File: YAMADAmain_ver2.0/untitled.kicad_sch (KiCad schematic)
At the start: 18 parts, among them J10 RX==RX, J11 TX==TX, J8 RX==TX, J9 TX==RX, U14 4.7k, U15 SW_DP3T, U16 0.1u, U18 STM32F446RETx-stm32, U19 0.1u, U20 0.1u, U22 0.1u, U23 0.1u, U3 0.1u, U4 D_Schottky, U7 4.7u, U9 ST-LINK

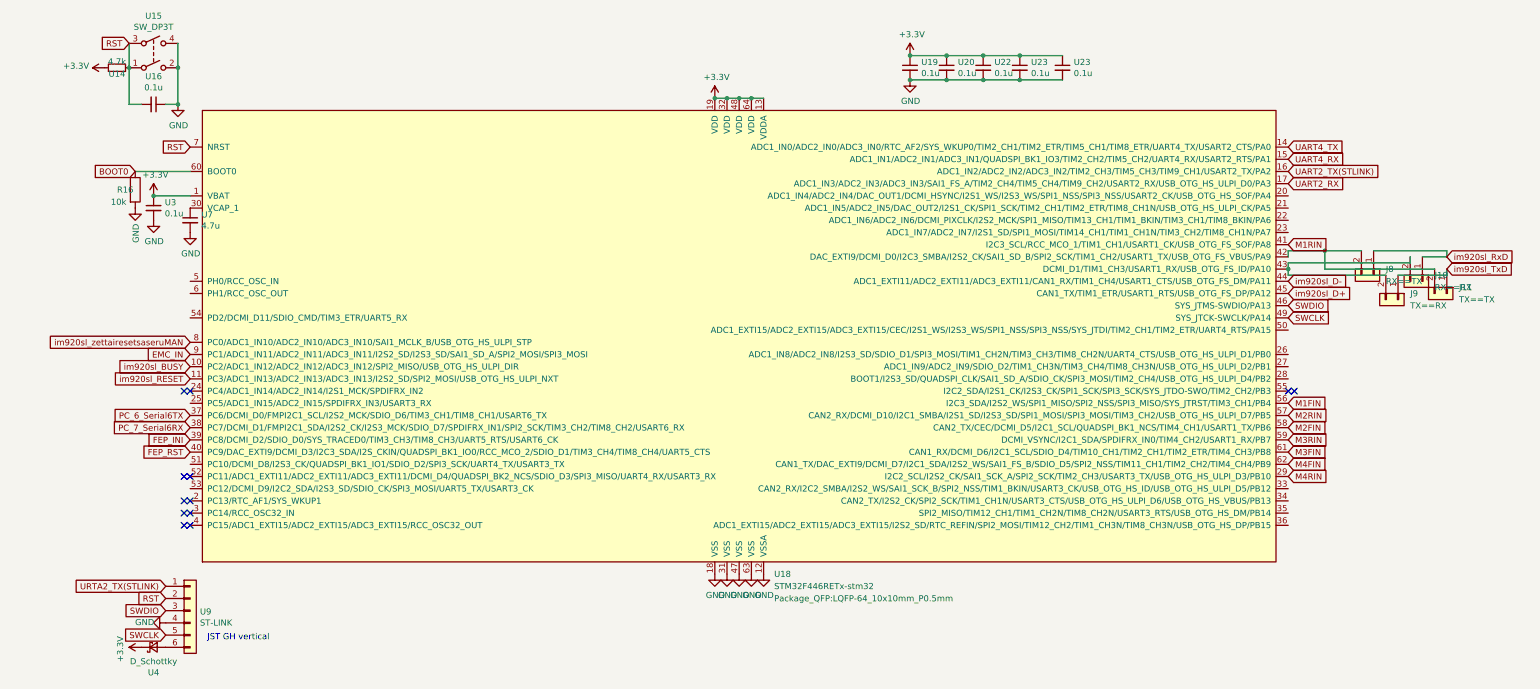
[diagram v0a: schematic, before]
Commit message: 2024/09/22
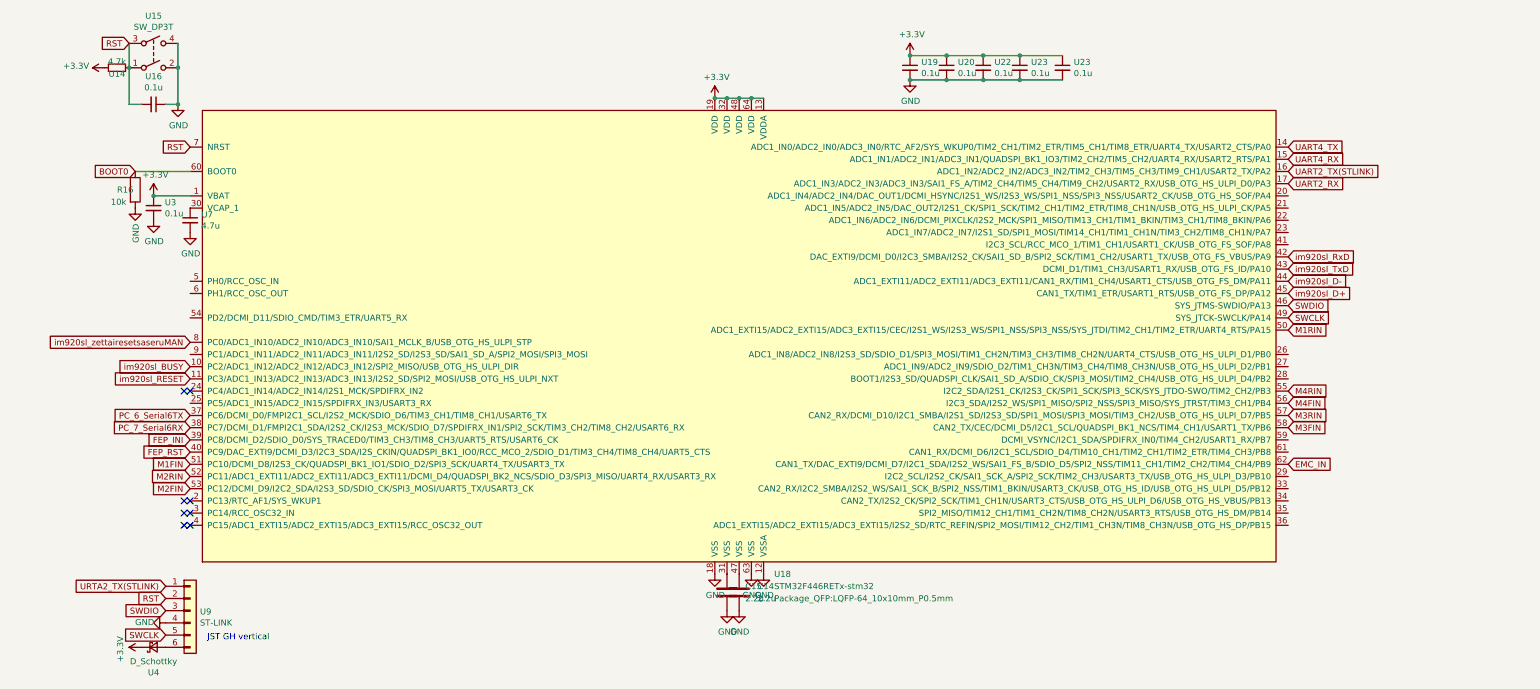
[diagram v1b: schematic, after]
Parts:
- removed J10: RX==RX, Jumper:SolderJumper-2_P1.3mm_Open_TrianglePad1.0x1.5mm, symbol Connector_Generic:Conn_01x02
- removed J11: TX==TX, Jumper:SolderJumper-2_P1.3mm_Open_TrianglePad1.0x1.5mm, symbol Connector_Generic:Conn_01x02
- removed J8: RX==TX, Jumper:SolderJumper-2_P1.3mm_Bridged_Pad1.0x1.5mm, symbol Connector_Generic:Conn_01x02
- removed J9: TX==RX, Jumper:SolderJumper-2_P1.3mm_Bridged_Pad1.0x1.5mm, symbol Connector_Generic:Conn_01x02
- added C14, C15: 2.2u, Footprint_nishi:C_0805_2012, symbol Device:C
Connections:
- net EMC_IN: now also U18.62 (CAN1_TX/DAC_EXTI9/DCMI_D7/I2C1_SDA/I2S2_WS/SAI1_FS_B/SDIO_D5/SPI2_NSS/TIM11_CH1/TIM2_CH2/TIM4_CH4/PB9); no longer U18.9 (PC1/ADC1_IN11/ADC2_IN11/ADC3_IN11/I2S2_SD/I2S3_SD/SAI1_SD_A/SPI2_MOSI/SPI3_MOSI)
- net GND: now also C14.2, C15.2; no longer U18.31 (VSS), U18.47 (VSS)
- net M1FIN: now also U18.51 (PC10/DCMI_D8/I2S3_CK/QUADSPI_BK1_IO1/SDIO_D2/SPI3_SCK/UART4_TX/USART3_TX); no longer U18.56 (I2C3_SDA/I2S2_WS/SPI1_MISO/SPI2_NSS/SPI3_MISO/SYS_JTRST/TIM3_CH1/PB4)
- net M1RIN: now also U18.50 (ADC1_EXTI15/ADC2_EXTI15/ADC3_EXTI15/CEC/I2S1_WS/I2S3_WS/SPI1_NSS/SPI3_NSS/SYS_JTDI/TIM2_CH1/TIM2_ETR/UART4_RTS/PA15); no longer U18.41 (I2C3_SCL/RCC_MCO_1/TIM1_CH1/USART1_CK/USB_OTG_FS_SOF/PA8)
- net M2FIN: now also U18.53 (PC12/DCMI_D9/I2C2_SDA/I2S3_SD/SDIO_CK/SPI3_MOSI/UART5_TX/USART3_CK); no longer U18.58 (CAN2_TX/CEC/DCMI_D5/I2C1_SCL/QUADSPI_BK1_NCS/TIM4_CH1/USART1_TX/PB6)
- net M2RIN: now also U18.52 (PC11/ADC1_EXTI11/ADC2_EXTI11/ADC3_EXTI11/DCMI_D4/QUADSPI_BK2_NCS/SDIO_D3/SPI3_MISO/UART4_RX/USART3_RX); no longer U18.57 (CAN2_RX/DCMI_D10/I2C1_SMBA/I2S1_SD/I2S3_SD/SPI1_MOSI/SPI3_MOSI/TIM3_CH2/USB_OTG_HS_ULPI_D7/PB5)
- net M3FIN: now also U18.58 (CAN2_TX/CEC/DCMI_D5/I2C1_SCL/QUADSPI_BK1_NCS/TIM4_CH1/USART1_TX/PB6); no longer U18.61 (CAN1_RX/DCMI_D6/I2C1_SCL/SDIO_D4/TIM10_CH1/TIM2_CH1/TIM2_ETR/TIM4_CH3/PB8)
- net M3RIN: now also U18.57 (CAN2_RX/DCMI_D10/I2C1_SMBA/I2S1_SD/I2S3_SD/SPI1_MOSI/SPI3_MOSI/TIM3_CH2/USB_OTG_HS_ULPI_D7/PB5); no longer U18.59 (DCMI_VSYNC/I2C1_SDA/SPDIFRX_IN0/TIM4_CH2/USART1_RX/PB7)
- net M4FIN: now also U18.56 (I2C3_SDA/I2S2_WS/SPI1_MISO/SPI2_NSS/SPI3_MISO/SYS_JTRST/TIM3_CH1/PB4); no longer U18.62 (CAN1_TX/DAC_EXTI9/DCMI_D7/I2C1_SDA/I2S2_WS/SAI1_FS_B/SDIO_D5/SPI2_NSS/TIM11_CH1/TIM2_CH2/TIM4_CH4/PB9)
- net M4RIN: now also U18.55 (I2C2_SDA/I2S1_CK/I2S3_CK/SPI1_SCK/SPI3_SCK/SYS_JTDO-SWO/TIM2_CH2/PB3); no longer U18.29 (I2C2_SCL/I2S2_CK/SAI1_SCK_A/SPI2_SCK/TIM2_CH3/USART3_TX/USB_OTG_HS_ULPI_D3/PB10)
- net im920sl_RxD: now also U18.42 (DAC_EXTI9/DCMI_D0/I2C3_SMBA/I2S2_CK/SAI1_SD_B/SPI2_SCK/TIM1_CH2/USART1_TX/USB_OTG_FS_VBUS/PA9)
- net im920sl_TxD: now also U18.43 (DCMI_D1/TIM1_CH3/USART1_RX/USB_OTG_FS_ID/PA10)
- new net: C15.1, U18.31 (VSS)
- new net: C14.1, U18.47 (VSS)
- no-connect marks 12 -> 8
